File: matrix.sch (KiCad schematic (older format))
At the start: 0 parts

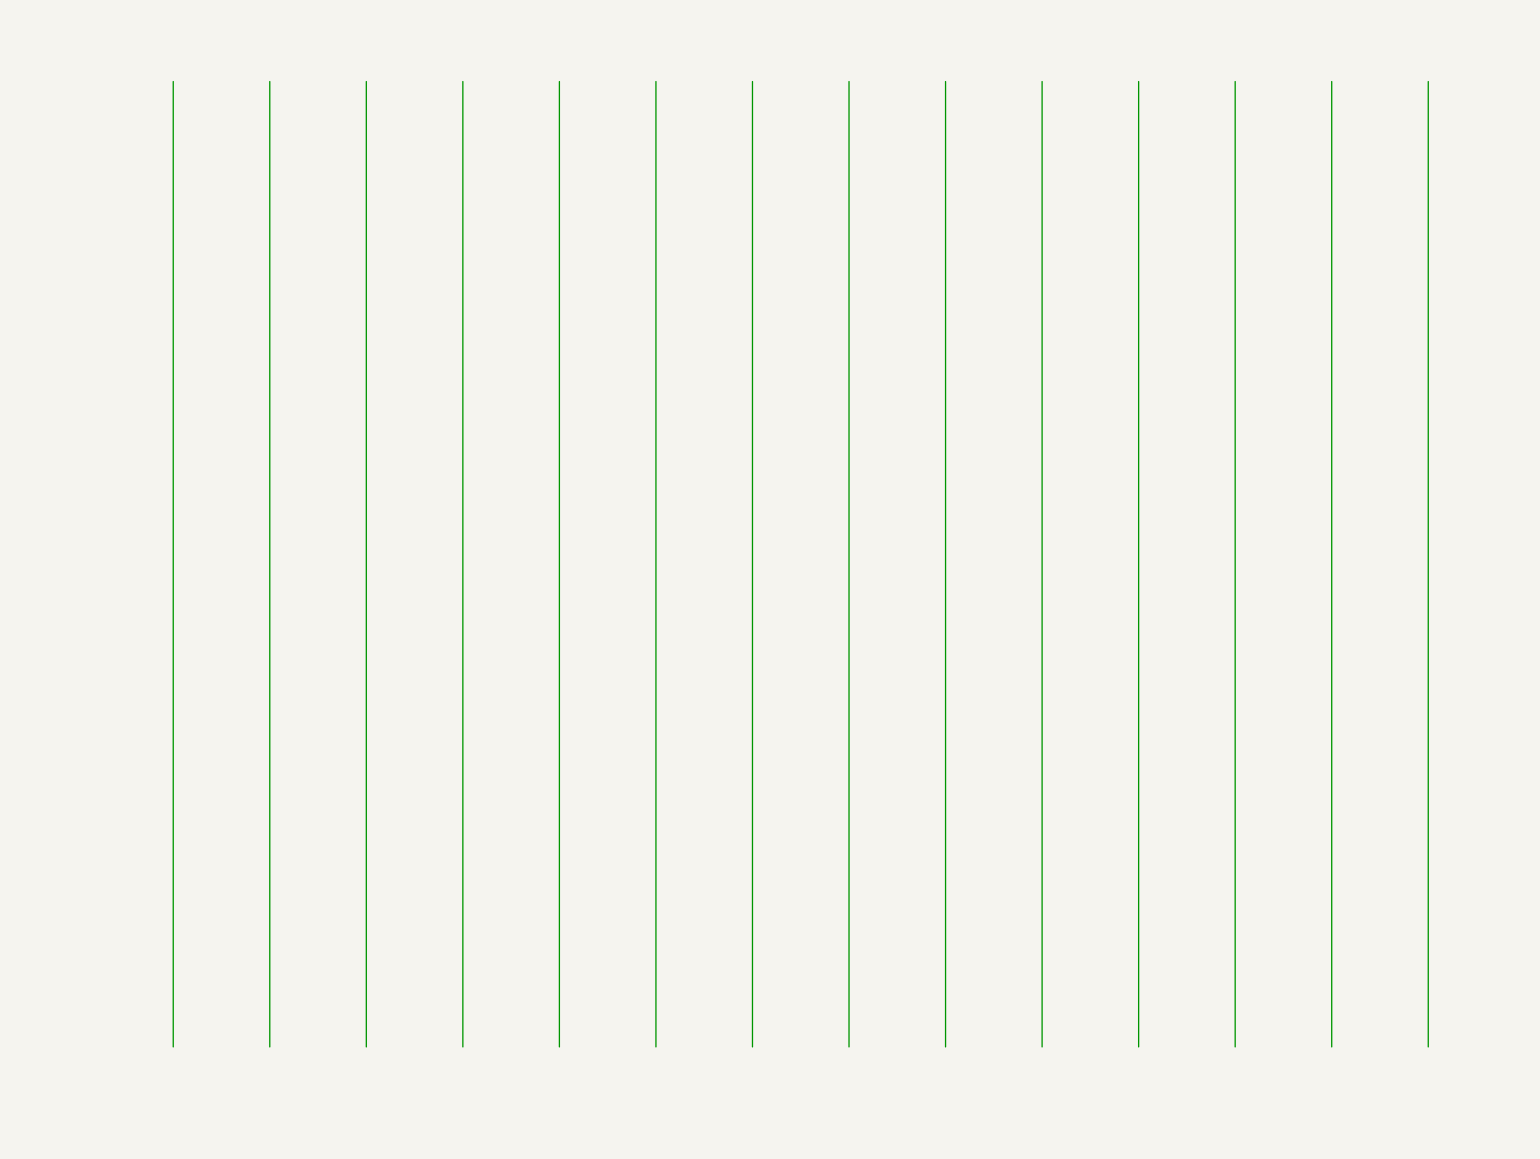
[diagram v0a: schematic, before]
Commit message: 20220311
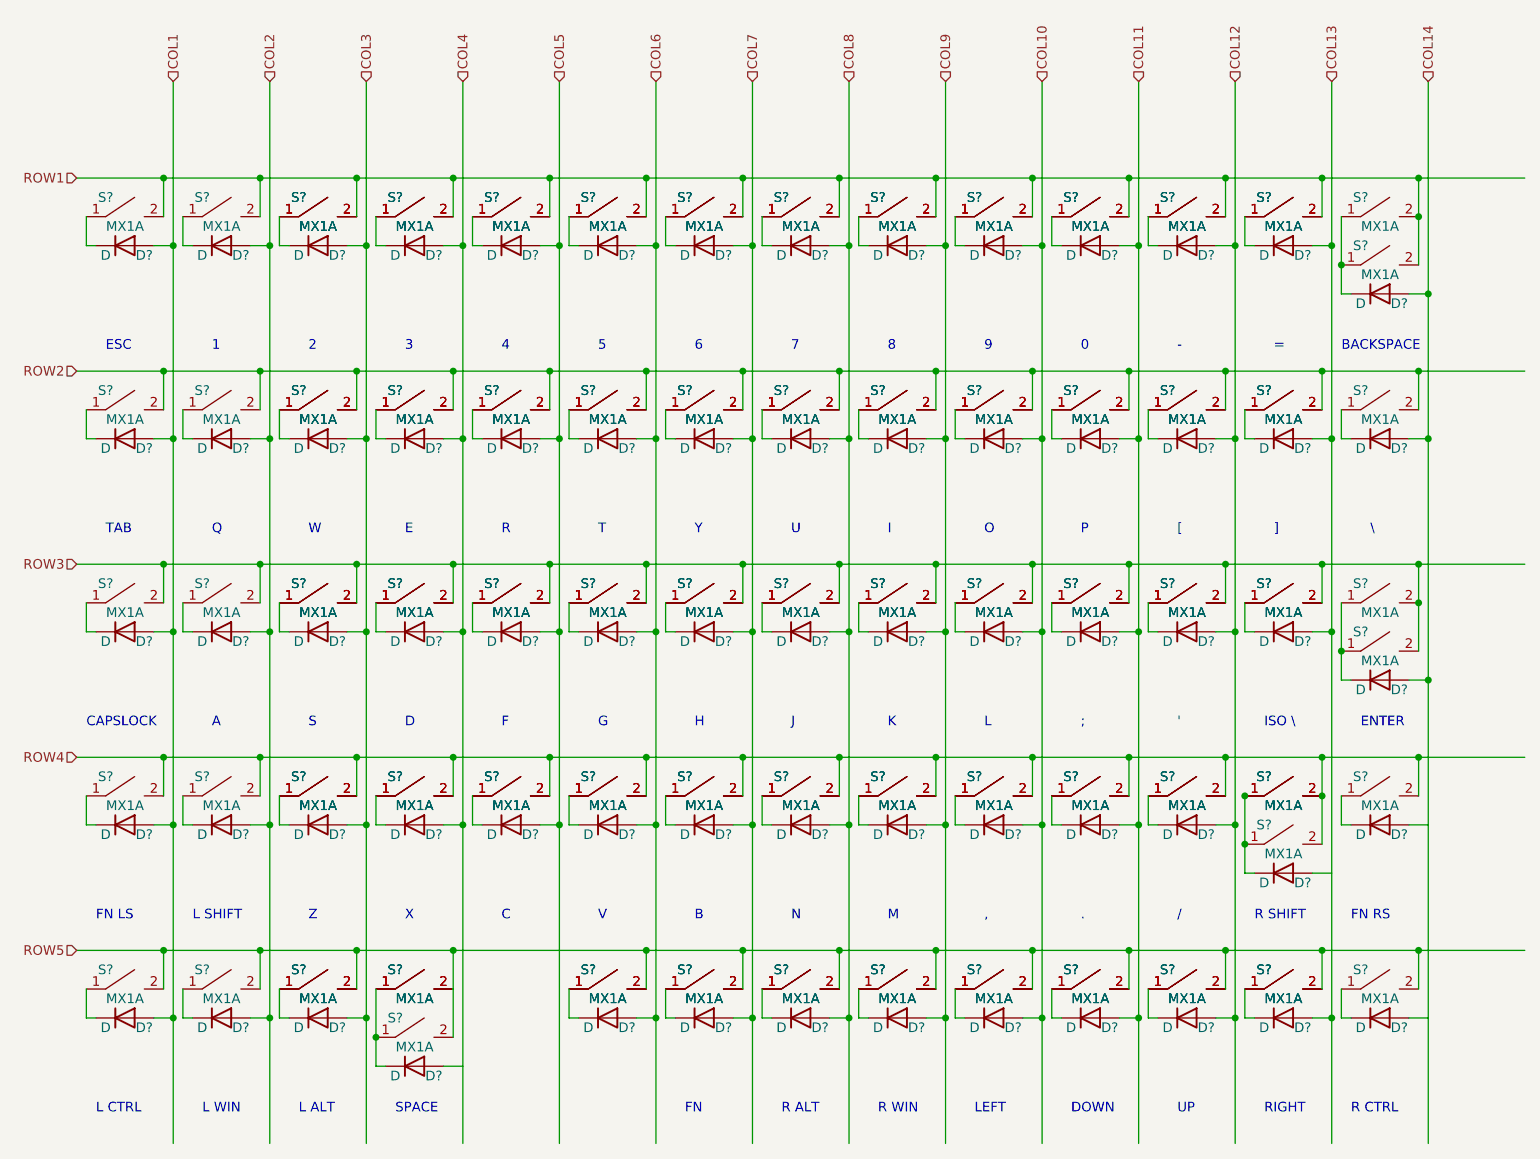
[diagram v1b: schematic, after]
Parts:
- added D? (x69): D, symbol Device:D
- added S? (x127): MX1A, symbol MX1A:MX1A
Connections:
- net labels added: COL1, COL10, COL11, COL12, COL13, COL14, COL2, COL3, COL4, COL5, COL6, COL7, COL8, COL9, ROW1, ROW2, ROW3, ROW4, ROW5
- wire segments 14 -> 437
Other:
- note added: "'"
- note added: ","
- note added: "-"
- note added: "."
- note added: "/"
- note added: "0"
- note added: "1"
- note added: "2"
- note added: "3"
- note added: "4"
- note added: "5"
- note added: "6"
- note added: "7"
- note added: "8"
- note added: "9"
- note added: ";"
- note added: "="
- note added: "A"
- note added: "B"
- note added: "BACKSPACE"
- note added: "C"
- note added: "CAPSLOCK"
- note added: "D"
- note added: "DOWN"
- note added: "E"
- note added: "ENTER"
- note added: "ESC"
- note added: "F"
- note added: "FN"
- note added: "FN LS"
- note added: "FN RS"
- note added: "G"
- note added: "H"
- note added: "I"
- note added: "ISO \"
- note added: "J"
- note added: "K"
- note added: "L"
- note added: "L ALT"
- note added: "L CTRL"
- note added: "L SHIFT"
- note added: "L WIN"
- note added: "LEFT"
- note added: "M"
- note added: "N"
- note added: "O"
- note added: "P"
- note added: "Q"
- note added: "R"
- note added: "R ALT"
- note added: "R CTRL"
- note added: "R SHIFT"
- note added: "R WIN"
- note added: "RIGHT"
- note added: "S"
- note added: "SPACE"
- note added: "T"
- note added: "TAB"
- note added: "U"
- note added: "UP"
- note added: "V"
- note added: "W"
- note added: "X"
- note added: "Y"
- note added: "Z"
- note added: "["
- note added: "\"
- note added: "]"
